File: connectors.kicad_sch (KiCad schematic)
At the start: 8 parts, among them CN102 EXPANSION, CN105 JOY1

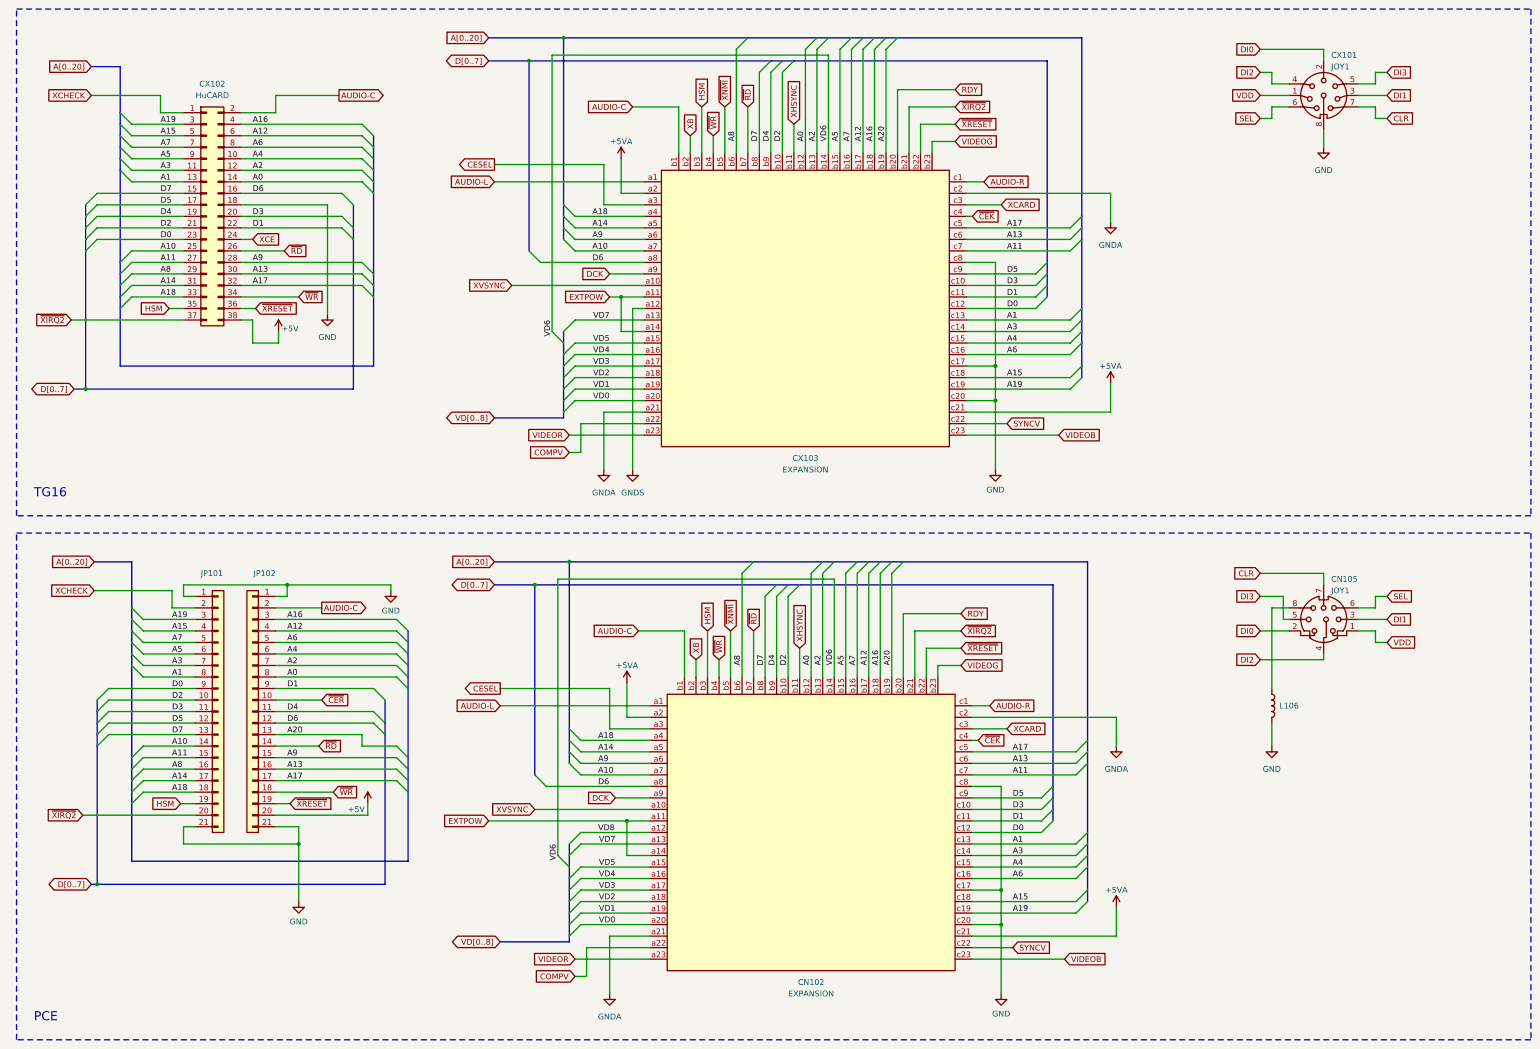
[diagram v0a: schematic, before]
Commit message: First draft of complete PCB.
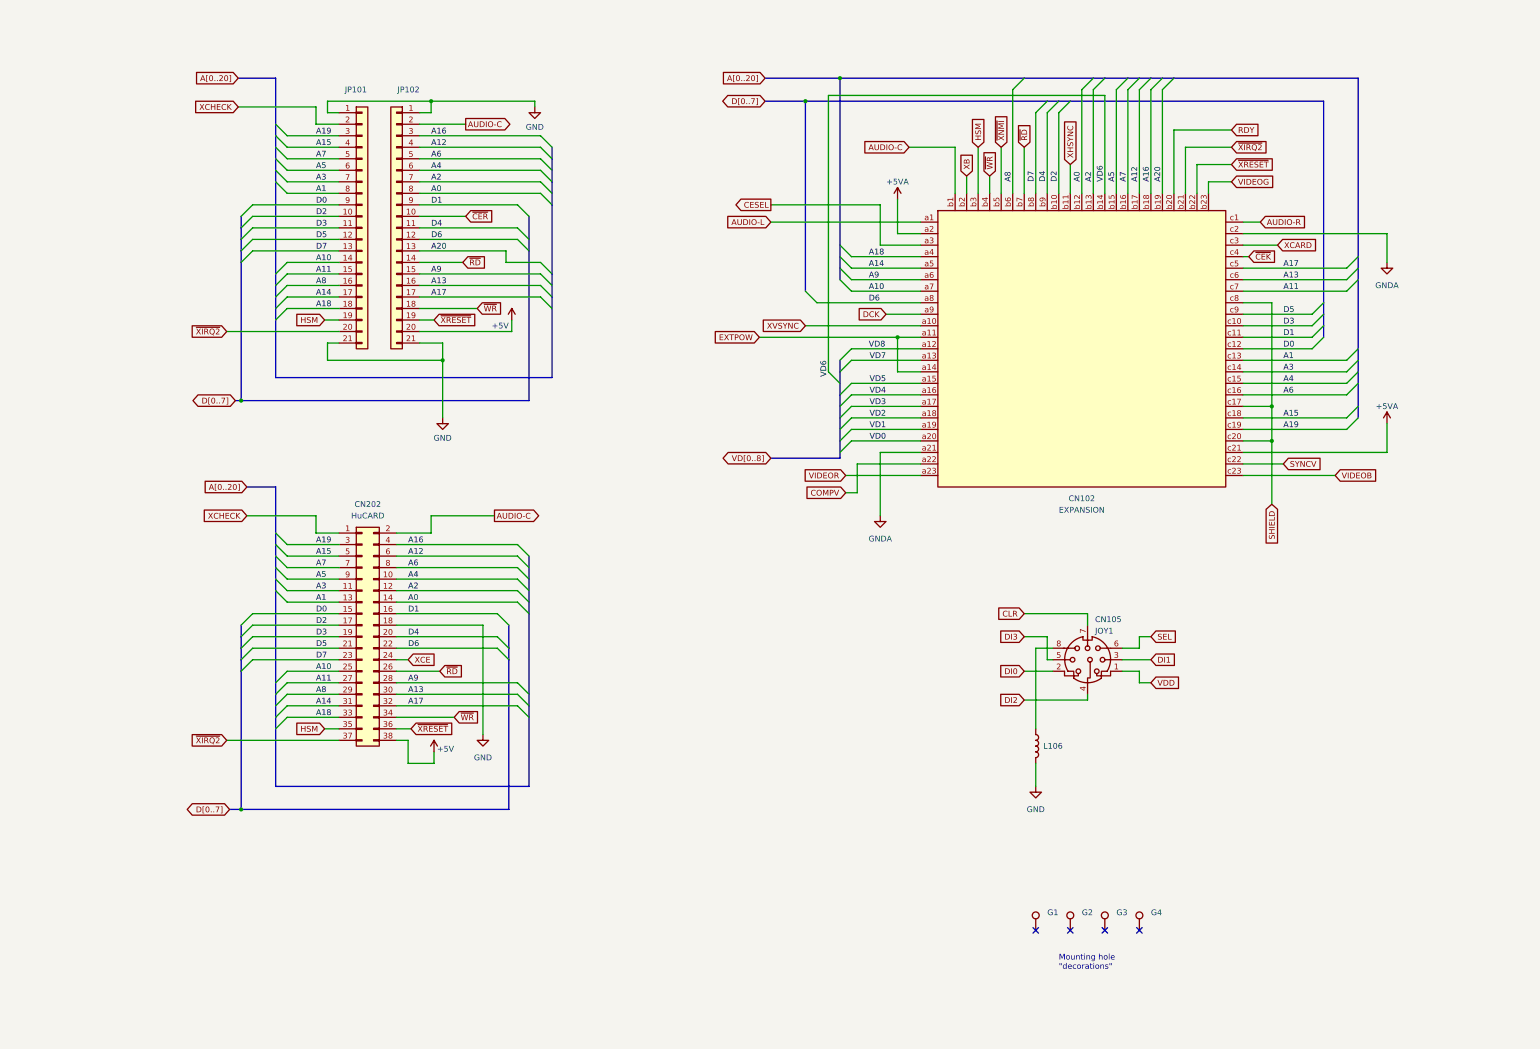
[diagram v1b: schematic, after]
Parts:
- removed CX101: JOY1, symbol Connector:DIN-8
- removed CX102: HuCARD, symbol Connector_Generic:Conn_02x19_Odd_Even
- removed CX103: EXPANSION, symbol PC-Engine:Conn_03x23
- added CN202: HuCARD, symbol Connector_Generic:Conn_02x19_Odd_Even
- added G1, G2, G3, G4: TestPoint, A-PCENGINE:Grounding_pad, symbol Connector:TestPoint
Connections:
- net +5V: now also CN202.38 (Pin_38)
- net A0: now also CN202.14 (Pin_14)
- net A1: now also CN202.13 (Pin_13)
- net A10: now also CN202.25 (Pin_25)
- net A11: now also CN202.27 (Pin_27)
- net A12: now also CN202.6 (Pin_6)
- net A13: now also CN202.30 (Pin_30)
- net A14: now also CN202.31 (Pin_31)
- net A15: now also CN202.5 (Pin_5)
- net A16: now also CN202.4 (Pin_4)
- net A17: now also CN202.32 (Pin_32)
- net A18: now also CN202.33 (Pin_33)
- net A19: now also CN202.3 (Pin_3)
- net A2: now also CN202.12 (Pin_12)
- net A3: now also CN202.11 (Pin_11)
- net A4: now also CN202.10 (Pin_10)
- net A5: now also CN202.9 (Pin_9)
- net A6: now also CN202.8 (Pin_8)
- net A7: now also CN202.7 (Pin_7)
- net A8: now also CN202.29 (Pin_29)
- net A9: now also CN202.28 (Pin_28)
- net AUDIO-C: now also CN202.2 (Pin_2)
- net D0: now also CN202.15 (Pin_15)
- net D1: now also CN202.16 (Pin_16)
- net D2: now also CN202.17 (Pin_17)
- net D3: now also CN202.19 (Pin_19)
- net D4: now also CN202.20 (Pin_20)
- net D5: now also CN202.21 (Pin_21)
- net D6: now also CN202.22 (Pin_22)
- net D7: now also CN202.23 (Pin_23)
- net GND: now also CN202.18 (Pin_18); no longer CN102.c17 (Pin_c17), CN102.c20 (Pin_c20), CN102.c8 (Pin_c8)
- net HSM: now also CN202.35 (Pin_35)
- net XCE: now also CN202.24 (Pin_24)
- net XCHECK: now also CN202.1 (Pin_1)
- net ~{RD}: now also CN202.26 (Pin_26)
- net ~{WR}: now also CN202.34 (Pin_34)
- net ~{XIRQ2}: now also CN202.37 (Pin_37)
- net ~{XRESET}: now also CN202.36 (Pin_36)
- new net SHIELD: CN102.c17 (Pin_c17), CN102.c20 (Pin_c20), CN102.c8 (Pin_c8)
- no-connect marks 0 -> 4
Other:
- note added: "Mounting hole "decorations""
- note removed: "PCE"
- note removed: "TG16"
- moved on the sheet: CN102, CN105, JP101, JP102, L106
